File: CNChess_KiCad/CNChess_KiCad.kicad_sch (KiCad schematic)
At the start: 30 parts, among them J1 Servomotor, J2 Barrel_Jack, J3 Motor1, J4 Motor2, J5 Fan, SW1 Limit switch 1, SW2 Limit switch 2, SW3 On/off switch, U1 ESP32C3

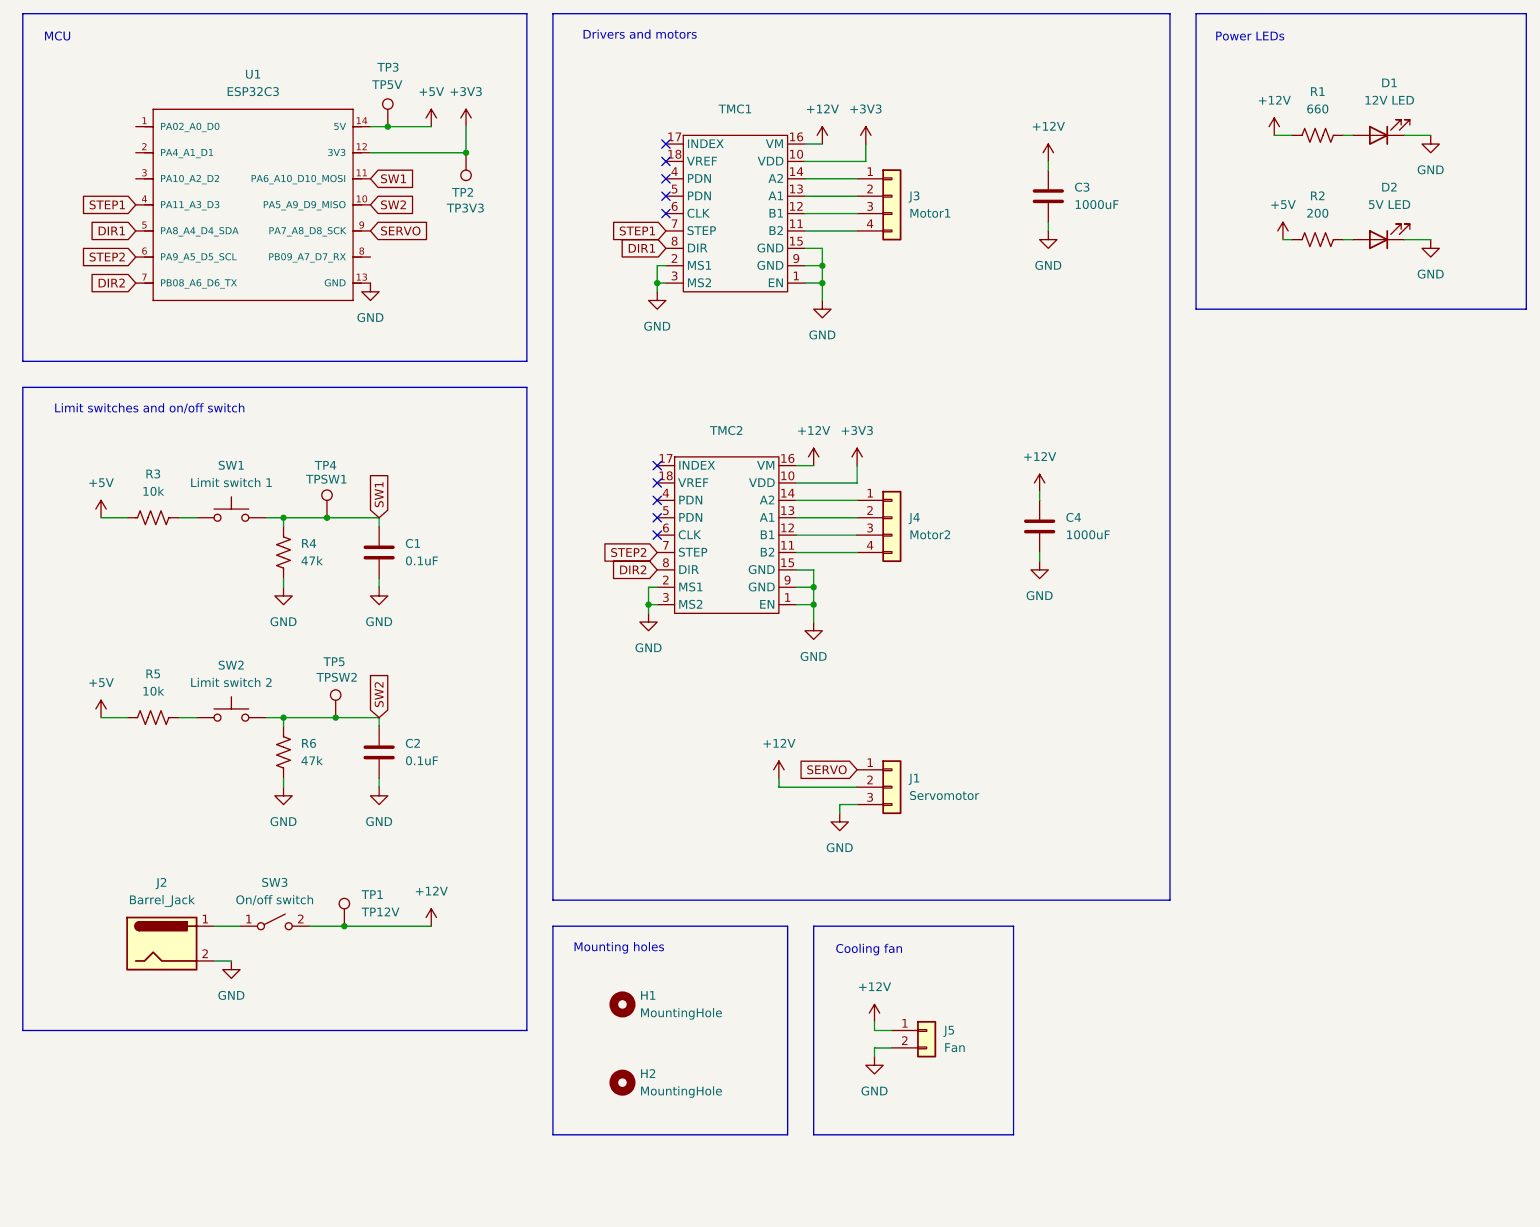
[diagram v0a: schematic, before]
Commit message: update kicad schematic
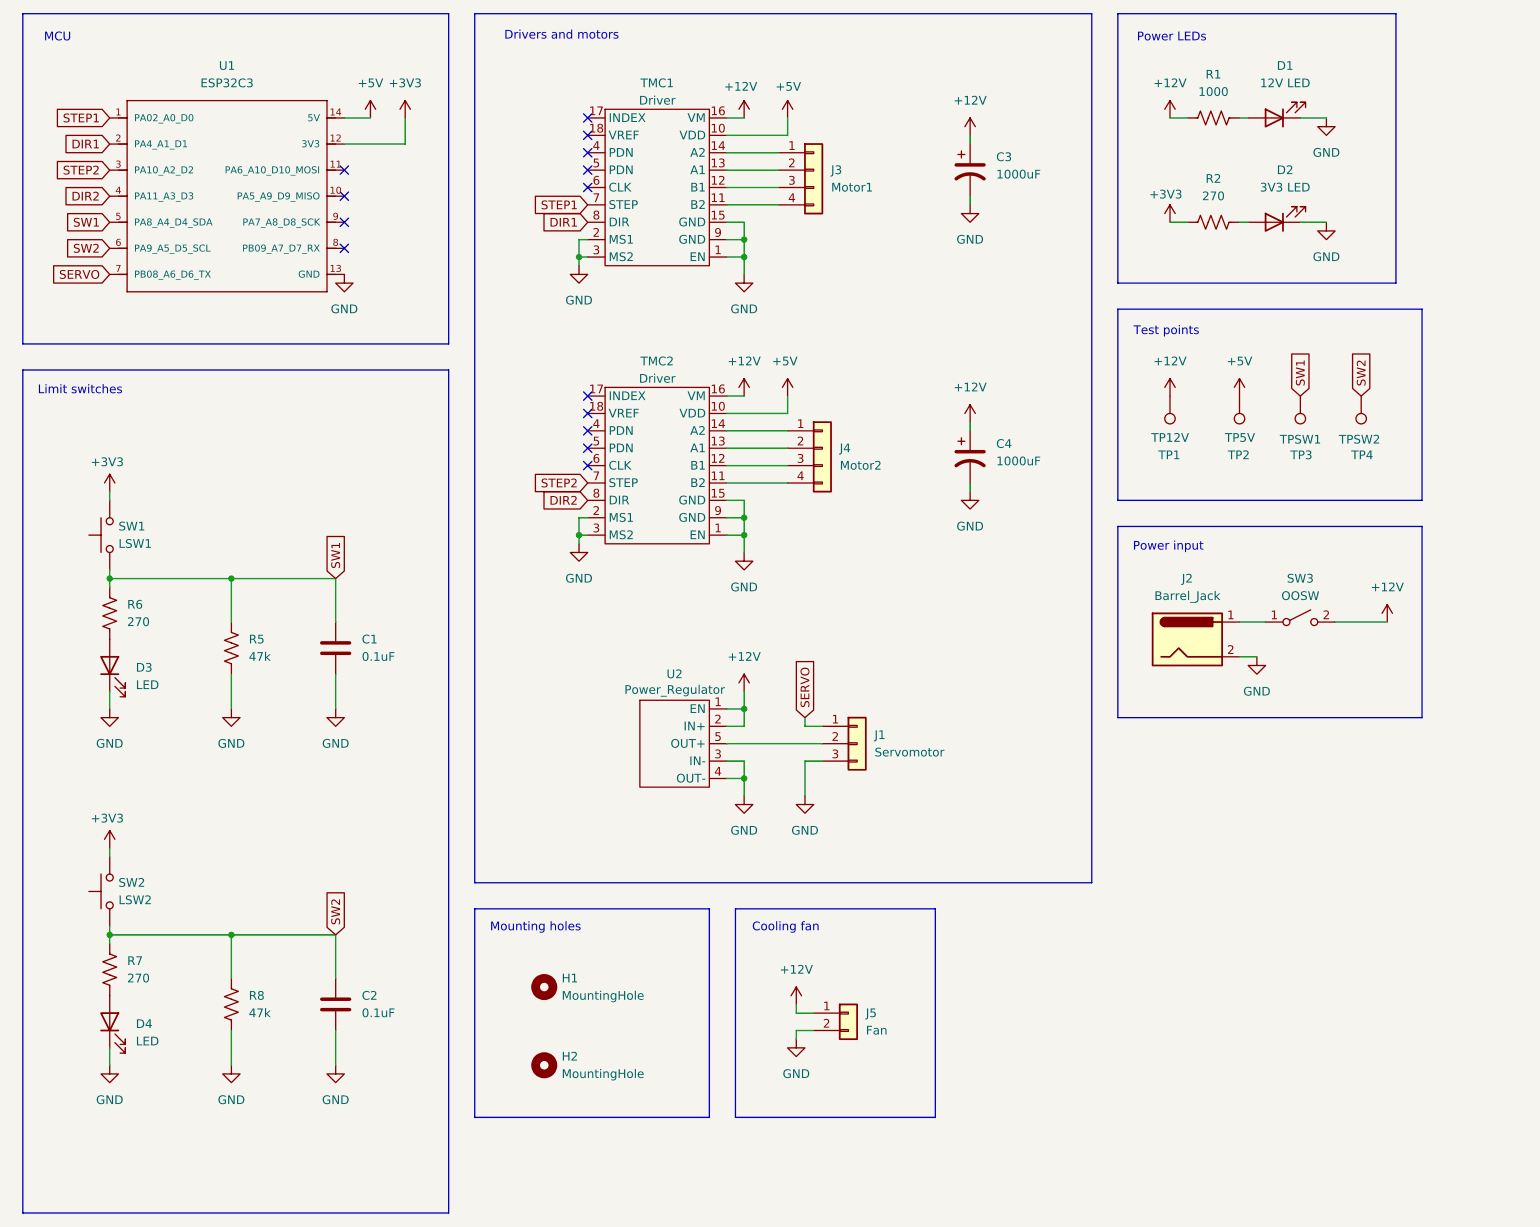
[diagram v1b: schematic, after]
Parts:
- removed C3, C4: 1000uF, symbol Device:C
- removed R3: 10k, symbol Device:R_US
- removed R4: 47k, symbol Device:R_US
- removed TP2: TP3V3, symbol Connector:TestPoint
- added C3, C4: 1000uF, Capacitor_THT:CP_Radial_D8.0mm_P3.50mm, symbol Device:C_Polarized_US
- added D3, D4: LED, Connector_JST:JST_XH_B2B-XH-A_1x02_P2.50mm_Vertical, symbol Device:LED
- added R7: 270, Resistor_THT:R_Axial_DIN0204_L3.6mm_D1.6mm_P5.08mm_Horizontal, symbol Device:R_US
- added R8: 47k, Resistor_THT:R_Axial_DIN0204_L3.6mm_D1.6mm_P5.08mm_Horizontal, symbol Device:R_US
- added U2: Power_Regulator, CNChess_footprints:Reg_12V, symbol CNChess:REG
- C1, C2: footprint (none) -> CNChess_footprints:CAP0_1u
- D1, J5: footprint (none) -> Connector_JST:JST_XH_B2B-XH-A_1x02_P2.50mm_Vertical
- D2: value 5V LED -> 3V3 LED; footprint (none) -> Connector_JST:JST_XH_B2B-XH-A_1x02_P2.50mm_Vertical
- H1, H2: footprint (none) -> MountingHole:MountingHole_3.2mm_M3_Pad
- J1: footprint (none) -> Connector_JST:JST_XH_B3B-XH-A_1x03_P2.50mm_Vertical
- J2: footprint (none) -> CNChess_footprints:BarrelJack_Horizontal
- J3, J4: footprint (none) -> Connector_JST:JST_XH_B4B-XH-A_1x04_P2.50mm_Vertical
- R1: value 660 -> 1000; footprint (none) -> Resistor_THT:R_Axial_DIN0204_L3.6mm_D1.6mm_P5.08mm_Horizontal
- R2: value 200 -> 270; footprint (none) -> Resistor_THT:R_Axial_DIN0204_L3.6mm_D1.6mm_P5.08mm_Horizontal
- R5: value 10k -> 47k; footprint (none) -> Resistor_THT:R_Axial_DIN0204_L3.6mm_D1.6mm_P5.08mm_Horizontal
- R6: value 47k -> 270; footprint (none) -> Resistor_THT:R_Axial_DIN0204_L3.6mm_D1.6mm_P5.08mm_Horizontal
- SW1: value Limit switch 1 -> LSW1; footprint (none) -> Connector_JST:JST_XH_B2B-XH-A_1x02_P2.50mm_Vertical
- SW2: value Limit switch 2 -> LSW2; footprint (none) -> Connector_JST:JST_XH_B2B-XH-A_1x02_P2.50mm_Vertical
- SW3: value On/off switch -> OOSW; footprint (none) -> Connector_JST:JST_XH_B2B-XH-A_1x02_P2.50mm_Vertical
- TMC1, TMC2: value ~ -> Driver; footprint TMC2209_footprint:TMC2209_header -> CNChess_footprints:TMC2209
- TP1: footprint (none) -> TestPoint:TestPoint_Pad_D1.5mm
- TP2: renamed from TP3; footprint (none) -> TestPoint:TestPoint_Pad_D1.5mm
- TP3: renamed from TP4; footprint (none) -> TestPoint:TestPoint_Pad_D1.5mm
- TP4: renamed from TP5; footprint (none) -> TestPoint:TestPoint_Pad_D1.5mm
- U1: footprint TMC2209_footprint:Esp32-C3 -> CNChess_footprints:Esp32-C3
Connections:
- net +12V: now also C3.1, C4.1, U2.1 (EN), U2.2 (IN+); no longer J1.2 (Pin_2)
- net +3V3: now also R2.1, SW1.2, SW2.2; no longer TMC1.10 (VDD), TMC2.10 (VDD)
- net +5V: now also TMC1.10 (VDD), TMC2.10 (VDD); no longer R2.1, R5.1
- net DIR1: now also U1.2 (PA4_A1_D1); no longer U1.5 (PA8_A4_D4_SDA)
- net DIR2: now also U1.4 (PA11_A3_D3); no longer U1.7 (PB08_A6_D6_TX)
- net GND: now also R5.1, C3.2, C4.2, D3.1 (K), D4.1 (K), R8.1, U2.3 (IN-), U2.4 (OUT-); no longer R6.2
- net SERVO: now also U1.7 (PB08_A6_D6_TX); no longer U1.9 (PA7_A8_D8_SCK)
- net STEP1: now also U1.1 (PA02_A0_D0); no longer U1.4 (PA11_A3_D3)
- net STEP2: now also U1.3 (PA10_A2_D2); no longer U1.6 (PA9_A5_D5_SCL)
- net SW1: now also R5.2, R6.2, SW1.1, U1.5 (PA8_A4_D4_SDA); no longer SW1.2, U1.11 (PA6_A10_D10_MOSI)
- net SW2: now also SW2.1, U1.6 (PA9_A5_D5_SCL), R7.2, R8.2; no longer R6.1, SW2.2, U1.10 (PA5_A9_D9_MISO)
- new net: D4.2 (A), R7.1
- new net: D3.2 (A), R6.1
- new net: J1.2 (Pin_2), U2.5 (OUT+)
- no-connect marks 10 -> 14
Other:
- note added: "Limit switches"
- note added: "Power input"
- note added: "Test points"
- note removed: "Limit switches and on/off switch"
- moved on the sheet: C1, D1, D2, H1, H2, J2, J3, J4, J5, R1, R2, SW1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
